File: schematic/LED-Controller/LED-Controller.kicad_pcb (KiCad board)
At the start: 2 copper layers, 40 x 32 mm, 14 parts, among them J1 5V Power, J2 ICSP, J3 RCin, J4 Serial Connect, J5 TSW-102-08-L-T-RA, J6 TSW-102-08-L-T-RA, J7 TSW-102-08-L-T-RA, U1 PIC18F27Q43-xSO

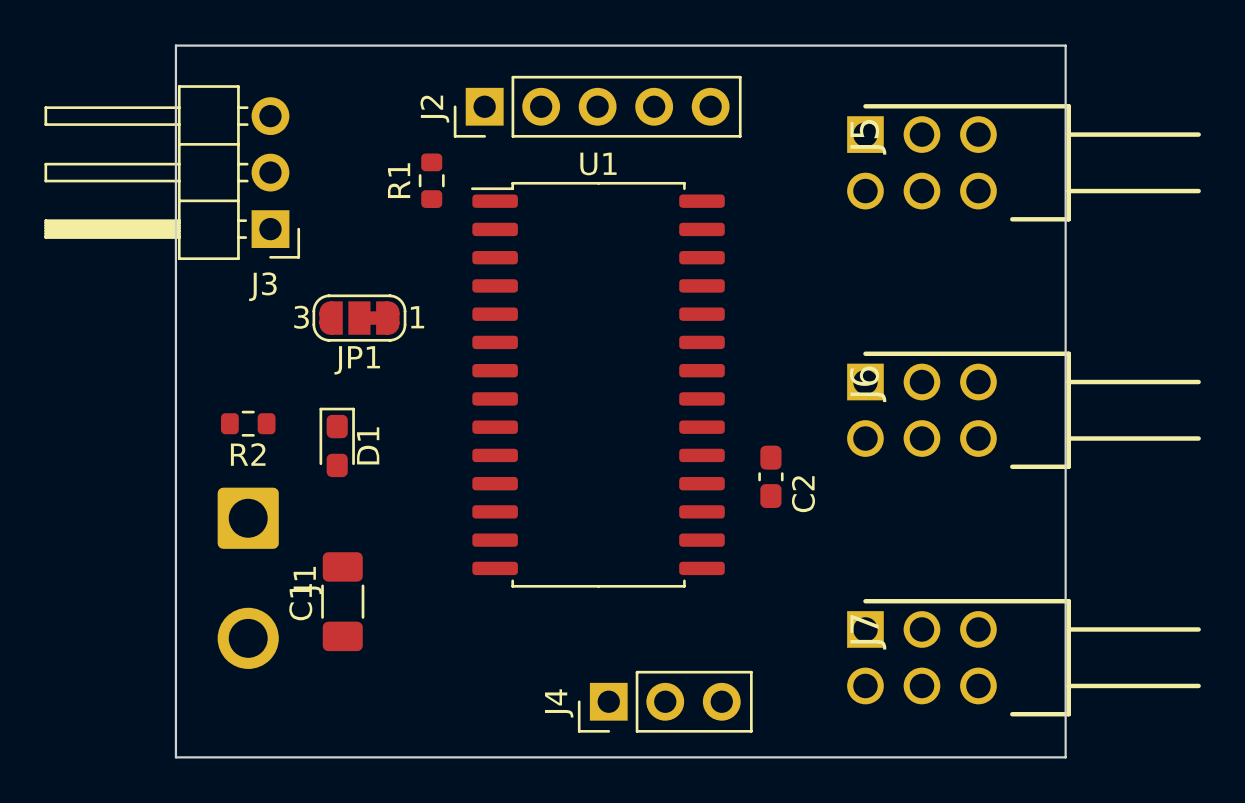
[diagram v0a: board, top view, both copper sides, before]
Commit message: Complete pcb layout
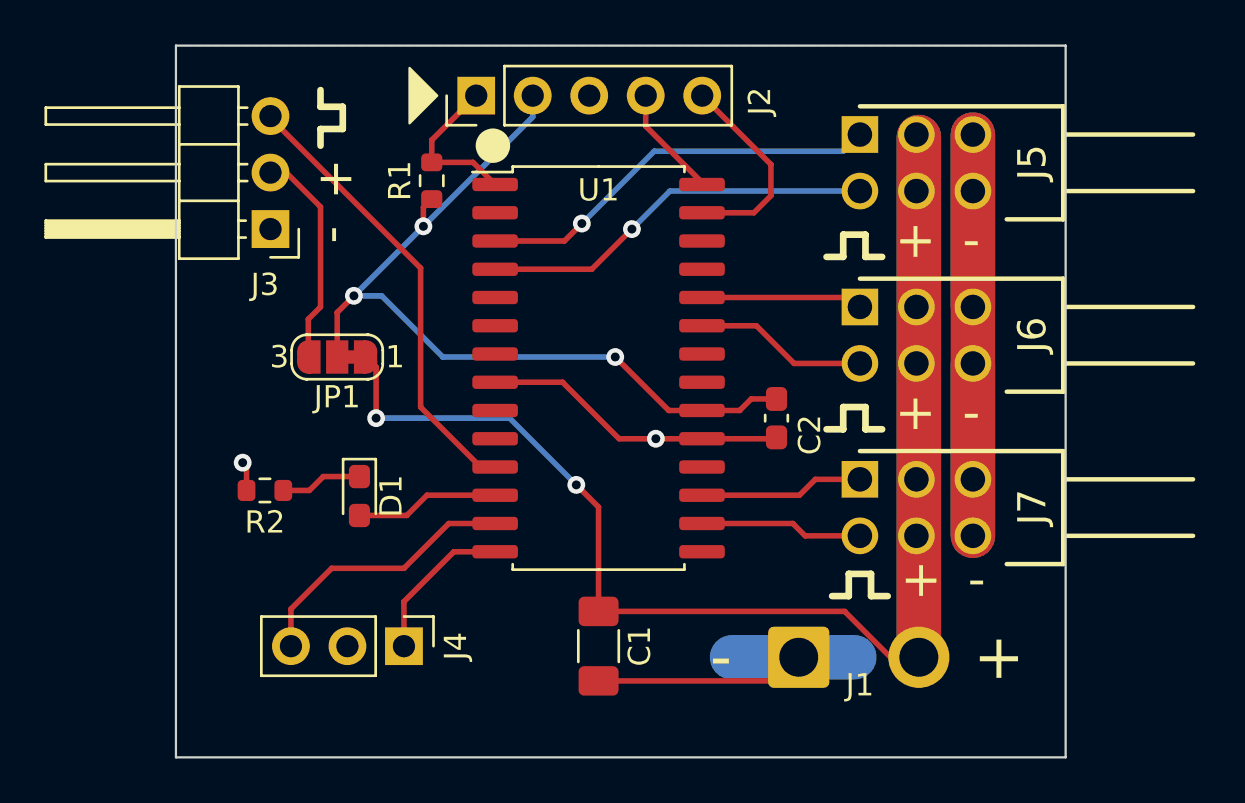
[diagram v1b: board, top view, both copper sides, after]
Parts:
- J5, J6, J7: value TSW-102-08-L-T-RA -> (none)
- moved J1 25.5 mm to (146.0, 97.0), turned to 0 degrees
- moved C1 11.7 mm to (137.0, 96.5), turned to 270 degrees
- moved J4 9.54 mm to (128.2, 96.5), turned to 270 degrees
- moved J7 6.75 mm to (148.8, 89.0)
- moved J6 3.38 mm to (148.8, 81.2)
- moved R2 3.09 mm to (122.0, 89.5)
- moved C2 2.65 mm to (145.0, 86.2)
- moved D1 2.46 mm to (126.2, 89.8)
- moved JP1 2.02 mm to (125.2, 83.5)
- moved U1 0.75 mm to (137.0, 84.0)
- moved J2 0.63 mm to (131.5, 71.8)
- moved J5 0.25 mm to (148.8, 73.5)
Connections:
- U1 pad 11: Net-(J4-Pad3) -> Net-(J3-Pad3)
- U1 pad 12: Net-(J4-Pad1) -> Net-(D1-Pad2)
- U1 pad 13: Net-(J3-Pad3) -> Net-(J4-Pad3)
- U1 pad 14: Net-(D1-Pad2) -> Net-(J4-Pad1)
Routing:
- net VDD: track 0.00 -> 81.6 mm, vias 0 -> 2
- net GND: track 0.00 -> 63.5 mm, vias 0 -> 2
- net /uC_Power: track 0.00 -> 38.1 mm, vias 0 -> 3
- net Net-(J3-Pad3): track 0.00 -> 20.3 mm
- net Net-(J5-Pad1): track 0.00 -> 18.4 mm, vias 0 -> 1
- net Net-(J5-Pad4): track 0.00 -> 17.9 mm, vias 0 -> 1
- net Net-(J4-Pad3): track 0.00 -> 12.4 mm
- net Net-(J3-Pad2): track 0.00 -> 9.87 mm
- net Net-(J2-Pad5): track 0.00 -> 9.20 mm
- net Net-(J6-Pad4): track 0.00 -> 7.80 mm
- net Net-(J7-Pad1): track 0.00 -> 7.40 mm
- net Net-(J7-Pad4): track 0.00 -> 7.33 mm
- net Net-(J6-Pad1): track 0.00 -> 7.28 mm
- net Net-(J2-Pad1): track 0.00 -> 7.09 mm
- net Net-(J4-Pad1): track 0.00 -> 7.03 mm
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- added copper zone on B.Cu, net GND
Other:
- board text added: "+"
- board text added: "-"
- board text added: "JLCJLCJLCJLC"
- board text added: "LED Controller"
- board text added: "QES 2021"
- board text added: "V 1.0"
